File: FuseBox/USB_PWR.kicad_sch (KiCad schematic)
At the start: 54 parts, among them J1 UJ31CHG2SMTTR, U1 TPS61040DBVR, U2 LT3030EFETRPBF

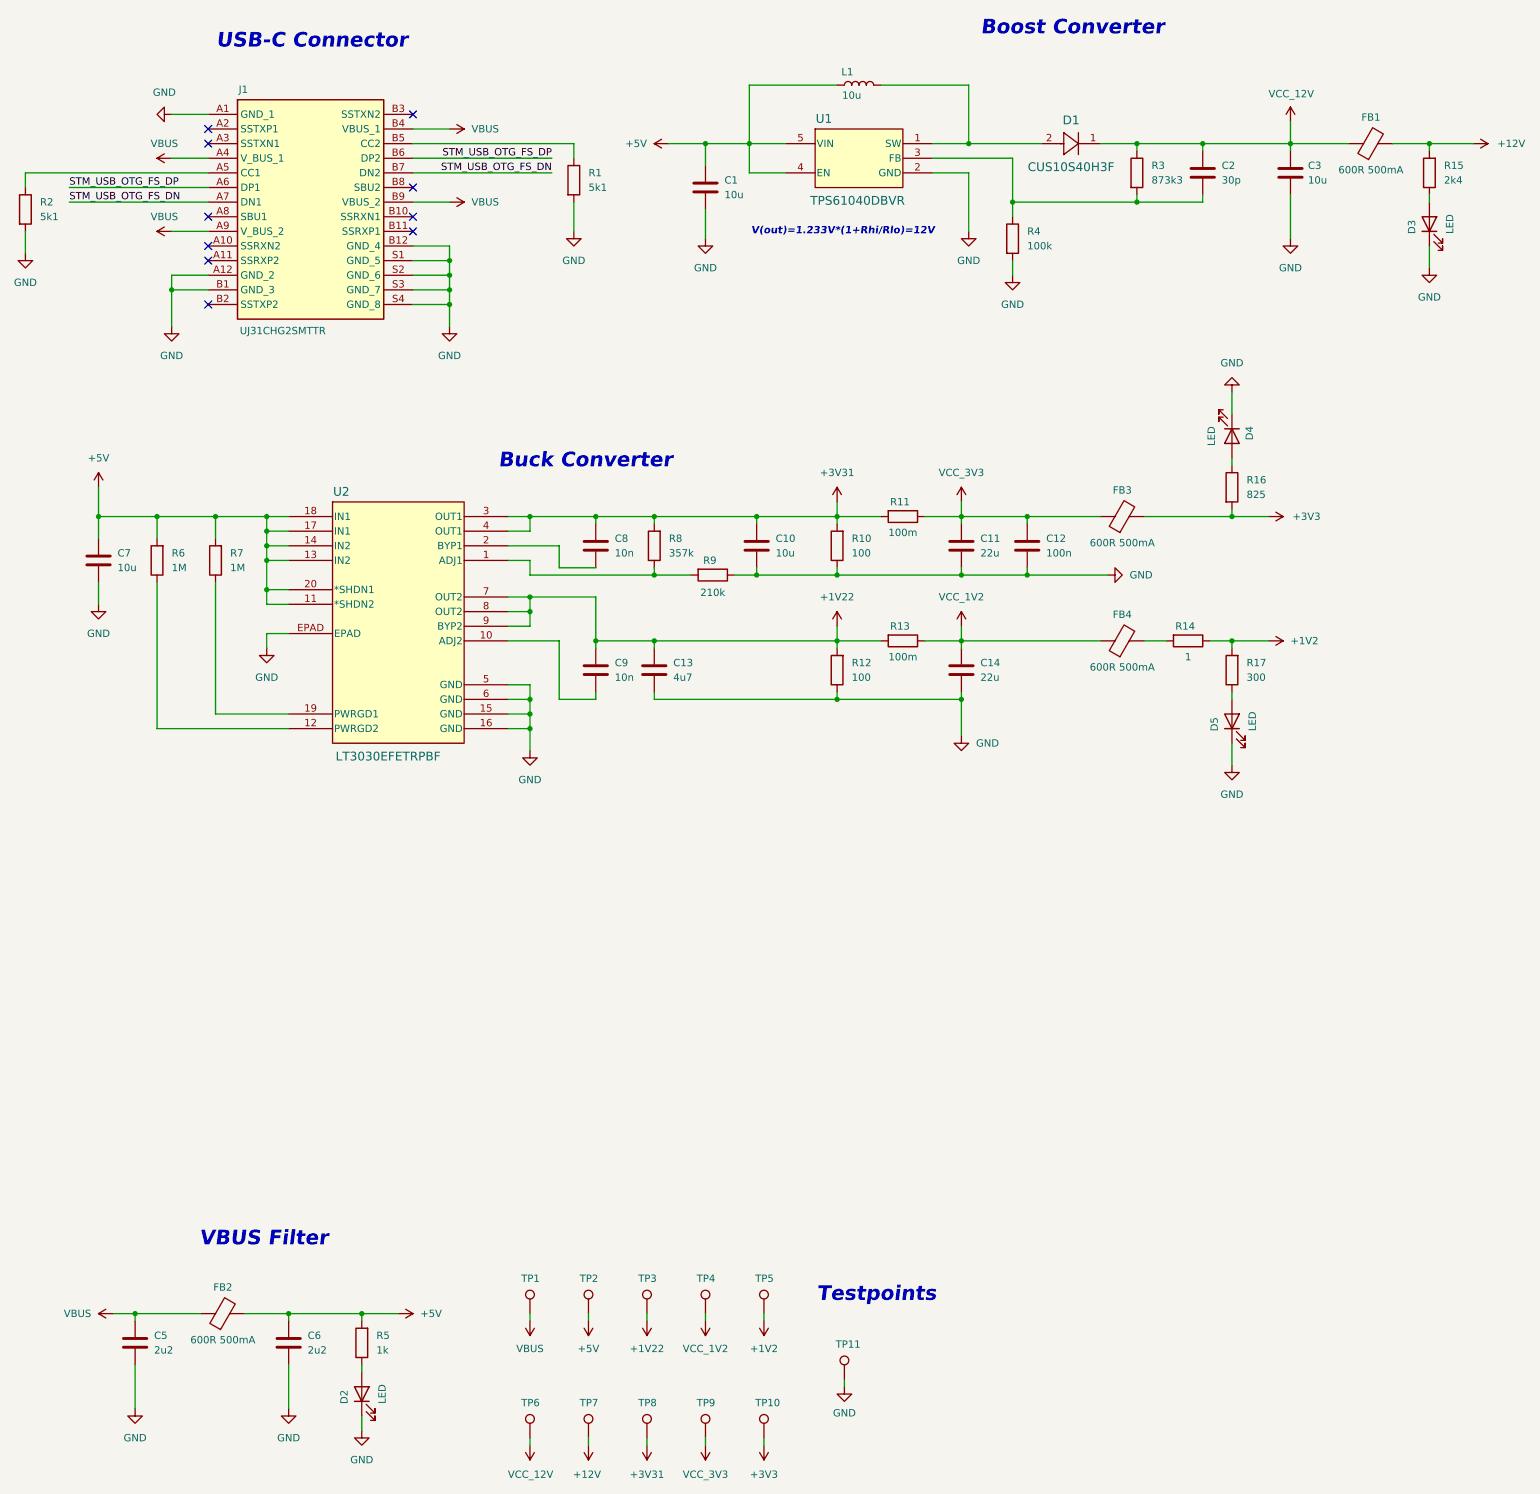
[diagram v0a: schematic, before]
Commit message: changuz
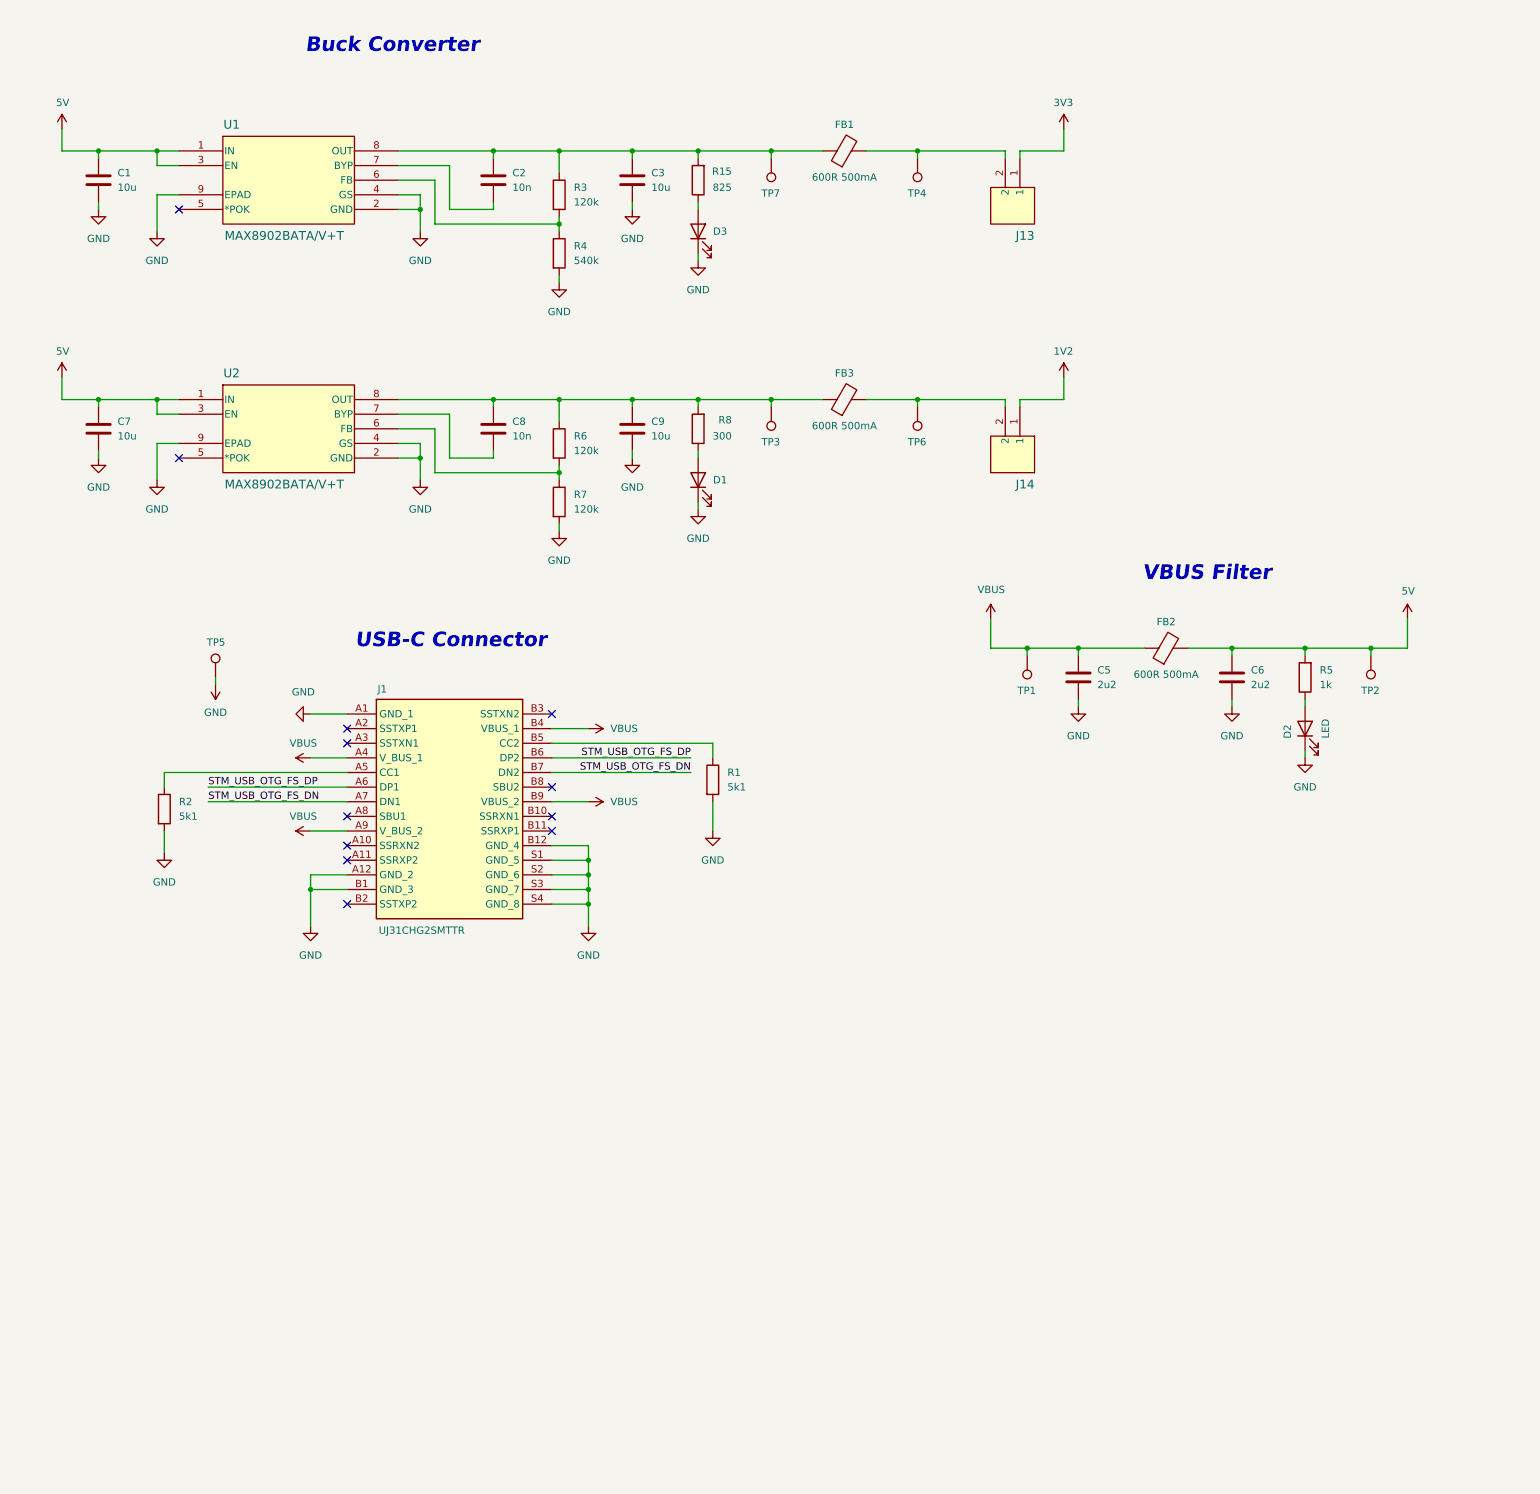
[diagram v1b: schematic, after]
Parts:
- removed C10: 10u, Capacitor_SMD:C_0603_1608Metric_Pad1.08x0.95mm_HandSolder, symbol Device:C
- removed C11, C14: 22u, Capacitor_SMD:C_0603_1608Metric_Pad1.08x0.95mm_HandSolder, symbol Device:C
- removed C12: 100n, Capacitor_SMD:C_0603_1608Metric_Pad1.08x0.95mm_HandSolder, symbol Device:C
- removed C13: 4u7, Capacitor_SMD:C_0603_1608Metric_Pad1.08x0.95mm_HandSolder, symbol Device:C
- removed D1: CUS10S40H3F, Custom:CUS10S40H3F, symbol Custom:CUS10S40H3F
- removed D3, D5: LED, LED_SMD:LED_0603_1608Metric, symbol Device:LED
- removed FB1, FB4: 600R 500mA, Inductor_SMD:L_0603_1608Metric_Pad1.05x0.95mm_HandSolder, symbol Device:FerriteBead
- removed L1: 10u, Inductor_SMD:L_0603_1608Metric_Pad1.05x0.95mm_HandSolder, symbol Device:L
- removed R10, R12: 100, Resistor_SMD:R_0603_1608Metric_Pad0.98x0.95mm_HandSolder, symbol Device:R
- removed R11, R13: 100m, Resistor_SMD:R_0603_1608Metric_Pad0.98x0.95mm_HandSolder, symbol Device:R
- removed R14: 1, Resistor_SMD:R_0603_1608Metric_Pad0.98x0.95mm_HandSolder, symbol Device:R
- removed R15: 2k4, Resistor_SMD:R_0603_1608Metric_Pad0.98x0.95mm_HandSolder, symbol Device:R
- removed R17: 300, Resistor_SMD:R_0603_1608Metric_Pad0.98x0.95mm_HandSolder, symbol Device:R
- removed R9: 210k, Resistor_SMD:R_0603_1608Metric_Pad0.98x0.95mm_HandSolder, symbol Device:R
- removed TP10, TP11, TP7, TP8, TP9: TestPoint, TestPoint:TestPoint_Pad_D3.0mm, symbol Connector:TestPoint
- removed U1: TPS61040DBVR, Custom:TPS61040DBVR, symbol Custom:TPS61040DBVR
- removed U2: LT3030EFETRPBF, Custom:LT8302ES8ETRPBF, symbol Custom:LT3030EFETRPBF
- added D1: LED, LED_SMD:LED_0603_1608Metric, symbol Device:LED
- added FB2: 600R 500mA, Inductor_SMD:L_0603_1608Metric_Pad1.05x0.95mm_HandSolder, symbol Device:FerriteBead
- added J13, J14: 61300211121, Custom:61300211121, symbol Custom:61300211121
- added TP4: TestPoint, TestPoint:TestPoint_Pad_D3.0mm, symbol Connector:TestPoint
- added U1, U2: MAX8902BATA/V+T, Custom:MAX8902BATAVT, symbol Custom:MAX8902BATAVT
- C2: value 30p -> 10n
- C9: value 10n -> 10u
- R3: value 873k3 -> 120k
- R4: value 100k -> 540k
- R6, R7: value 1M -> 120k
- R8: value 357k -> 300
- renumbered D4 to D3, FB2 to FB1, R16 to R15, TP4 to TP7
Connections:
- net +1V2 is gone; now on net GND: TP5.1
- net +1V22 is gone; now on an unnamed net: C9.1, TP3.1
- net +3V31 is gone; now on an unnamed net: C8.1, R8.2
- net VCC_1V2 is gone; now on an unnamed net: TP7.1
- net VCC_3V3 is gone; now on an unnamed net: FB3.1
- net GND: now also C9.2, R7.2, D1.1 (K), U1.2 (GND), U1.4 (GS), U1.9 (EPAD), U2.2 (GND), U2.4 (GS), U2.9 (EPAD)
- net VBUS: now also FB2.1; no longer FB1.1
- net at C8.2: now also U2.7 (BYP)
- net at R3.2, R4.1: now also U1.6 (FB); no longer C2.2
- net at R8.1: now also D1.2 (A)
- net at R6.1: now also U2.8 (OUT)
- net at R7.1: now also R6.2, U2.6 (FB)
- net +3V3: no longer names the net of R15.2
- net +3V3: now also C2.1, C3.1, FB1.1, R3.1, U1.8 (OUT); no longer FB3.2
- net +5V renamed 5V
- net 5V: now also FB2.2, U1.1 (IN), U1.3 (EN), U2.1 (IN), U2.3 (EN); no longer FB1.2, R6.2, R7.2
- removed net VCC_12V: C2.1, C3.1, R3.1, TP6.1
- new net: FB1.2, J13.2, TP4.1
- new net: FB3.2, J14.2, TP6.1
- new net: C2.2, U1.7 (BYP)
- new net 1V2: J14.1
- new net 3V3: J13.1
- no-connect marks 10 -> 12
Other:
- note removed: "Boost Converter"
- note removed: "Testpoints"
- note removed: "V(out)=1.233V*(1+Rhi/Rlo)=12V"
- moved on the sheet: C5, C6, D2, D3, FB1, J1, R1, R15, R2, R5, TP1, TP5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
